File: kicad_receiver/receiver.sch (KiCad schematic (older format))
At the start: 59 parts, among them J1 Conn_01x05_Male, J2 Conn_01x01, J3 Conn_01x01, J4 Conn_01x01, J5 Conn_01x01, J6 Conn_01x01, J7 Conn_01x01, U1 LP2985-3.3, U10 L9110, U11 4N26, U12 4N26, U2 LP2985-3.3, U3 STM32F030F4Px, U4 NRF24L01_Breakout, U5 TP4056, U6 L9110, U7 MT3608, U8 4N26, U9 4N26

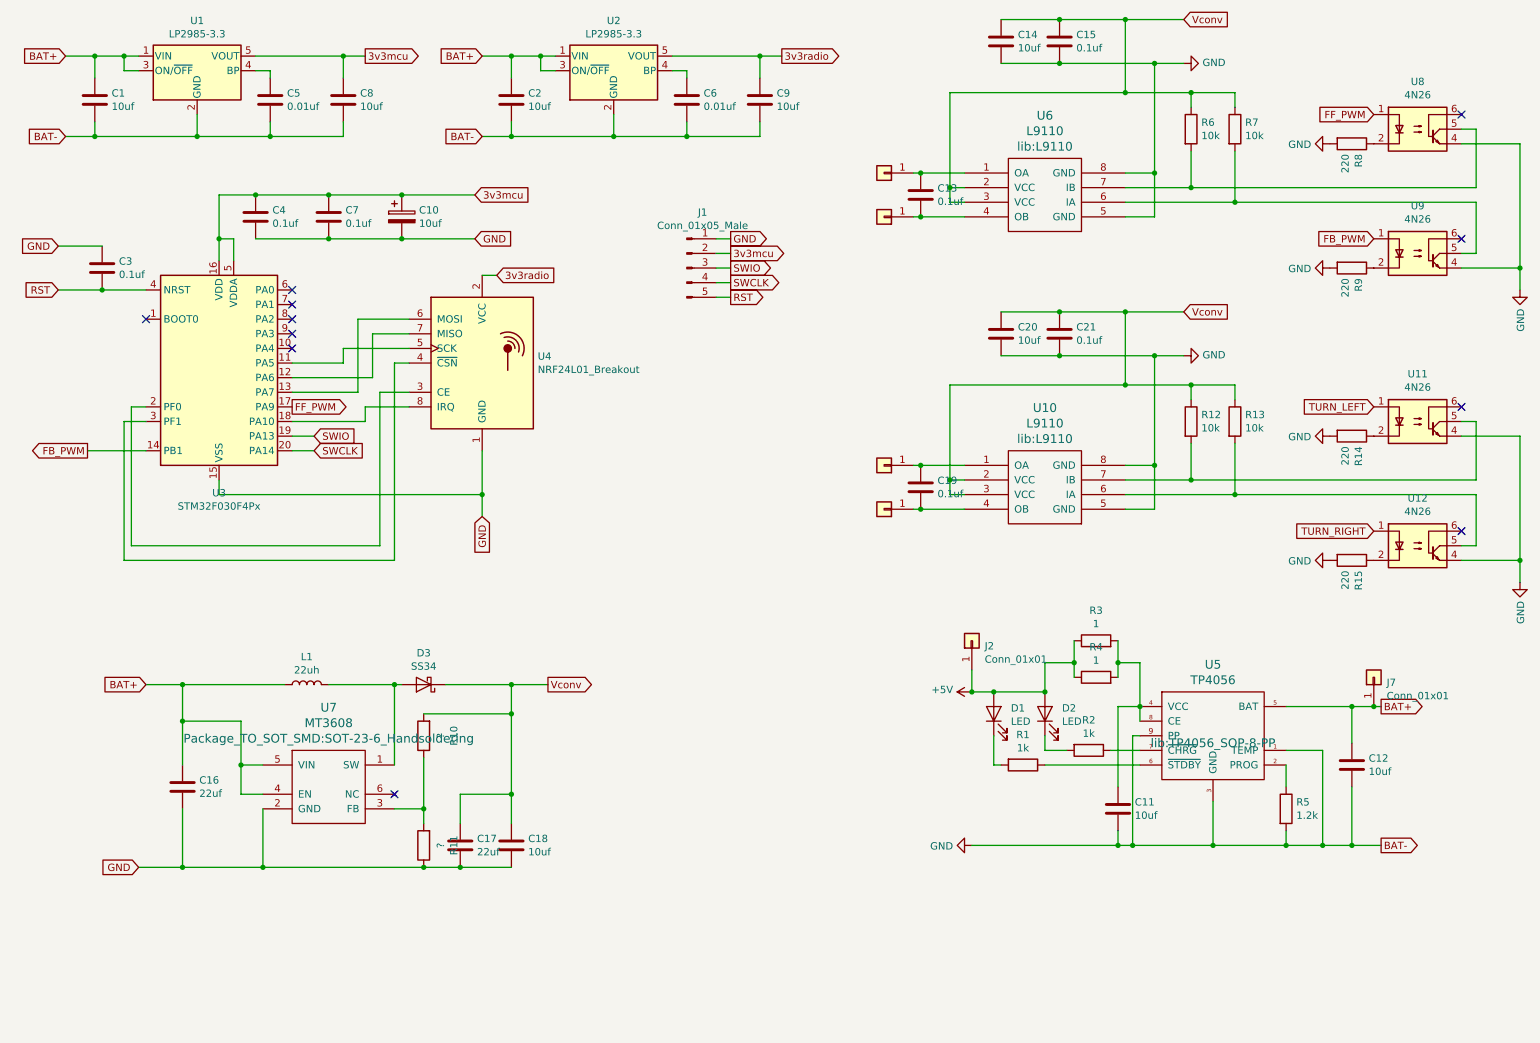
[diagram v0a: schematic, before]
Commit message: refactored
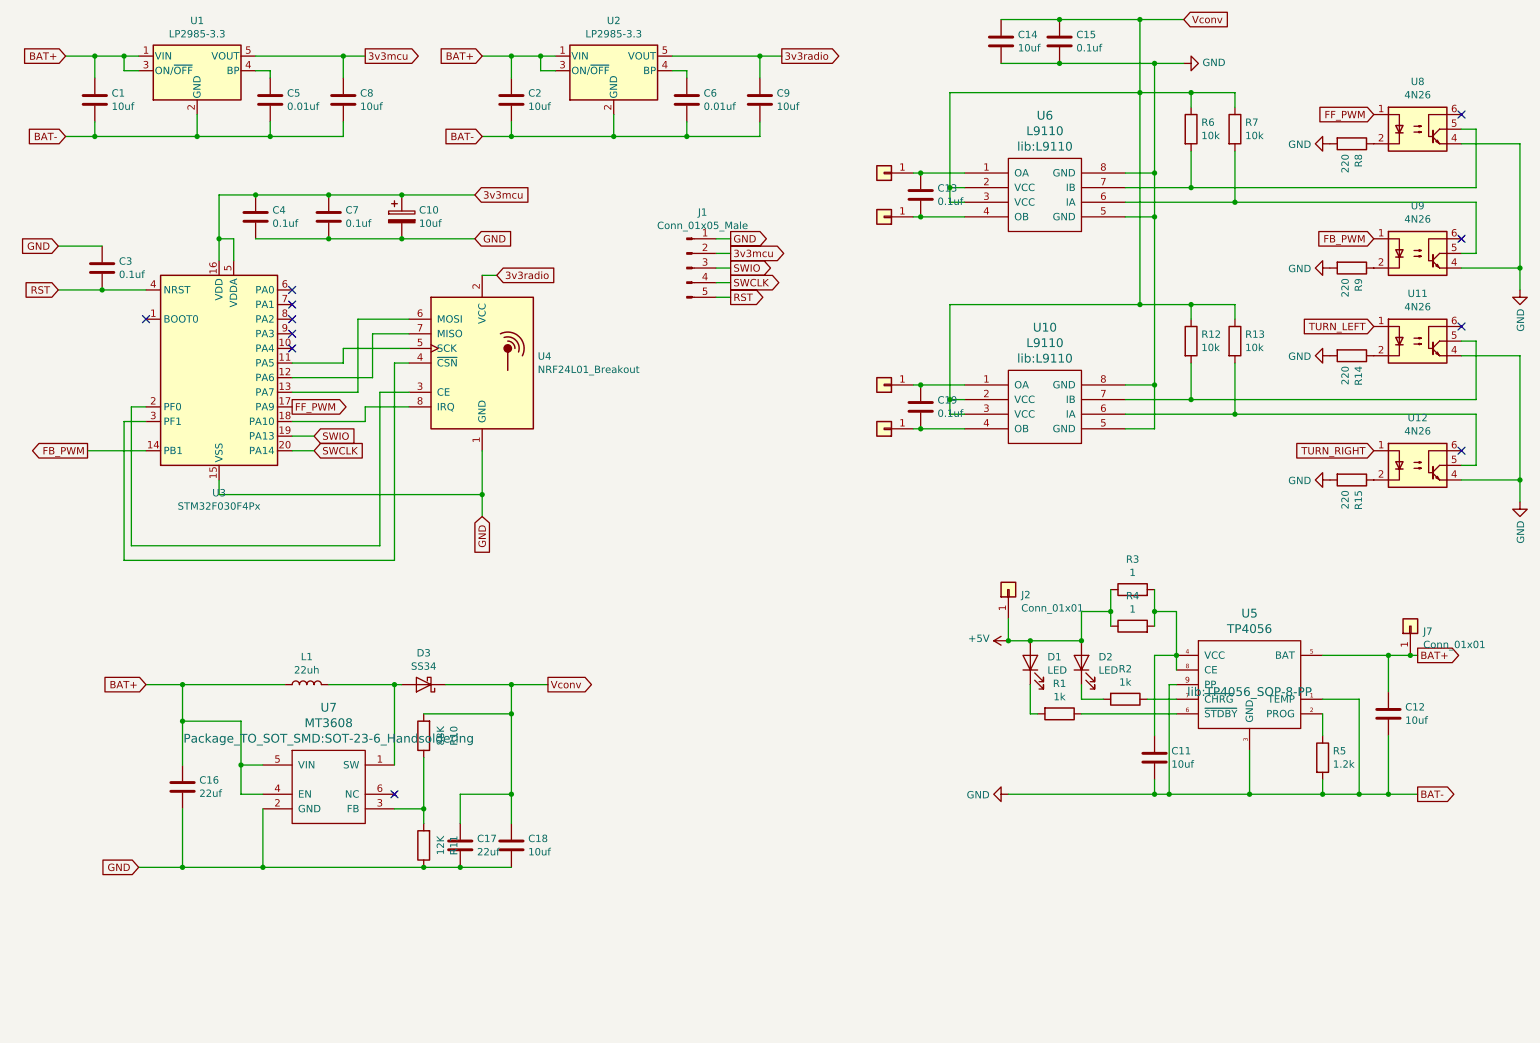
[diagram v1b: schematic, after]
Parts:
- removed C20: 10uf, Capacitor_SMD:C_0603_1608Metric_Pad1.05x0.95mm_HandSolder, symbol Device:C
- removed C21: 0.1uf, Capacitor_SMD:C_0603_1608Metric_Pad1.05x0.95mm_HandSolder, symbol Device:C
- R10: value ? -> 88K
- R11: value ? -> 12K
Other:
- moved on the sheet: C11, C12, C19, D1, D2, J2, J7, R1, R12, R13, R14, R15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

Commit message: place done
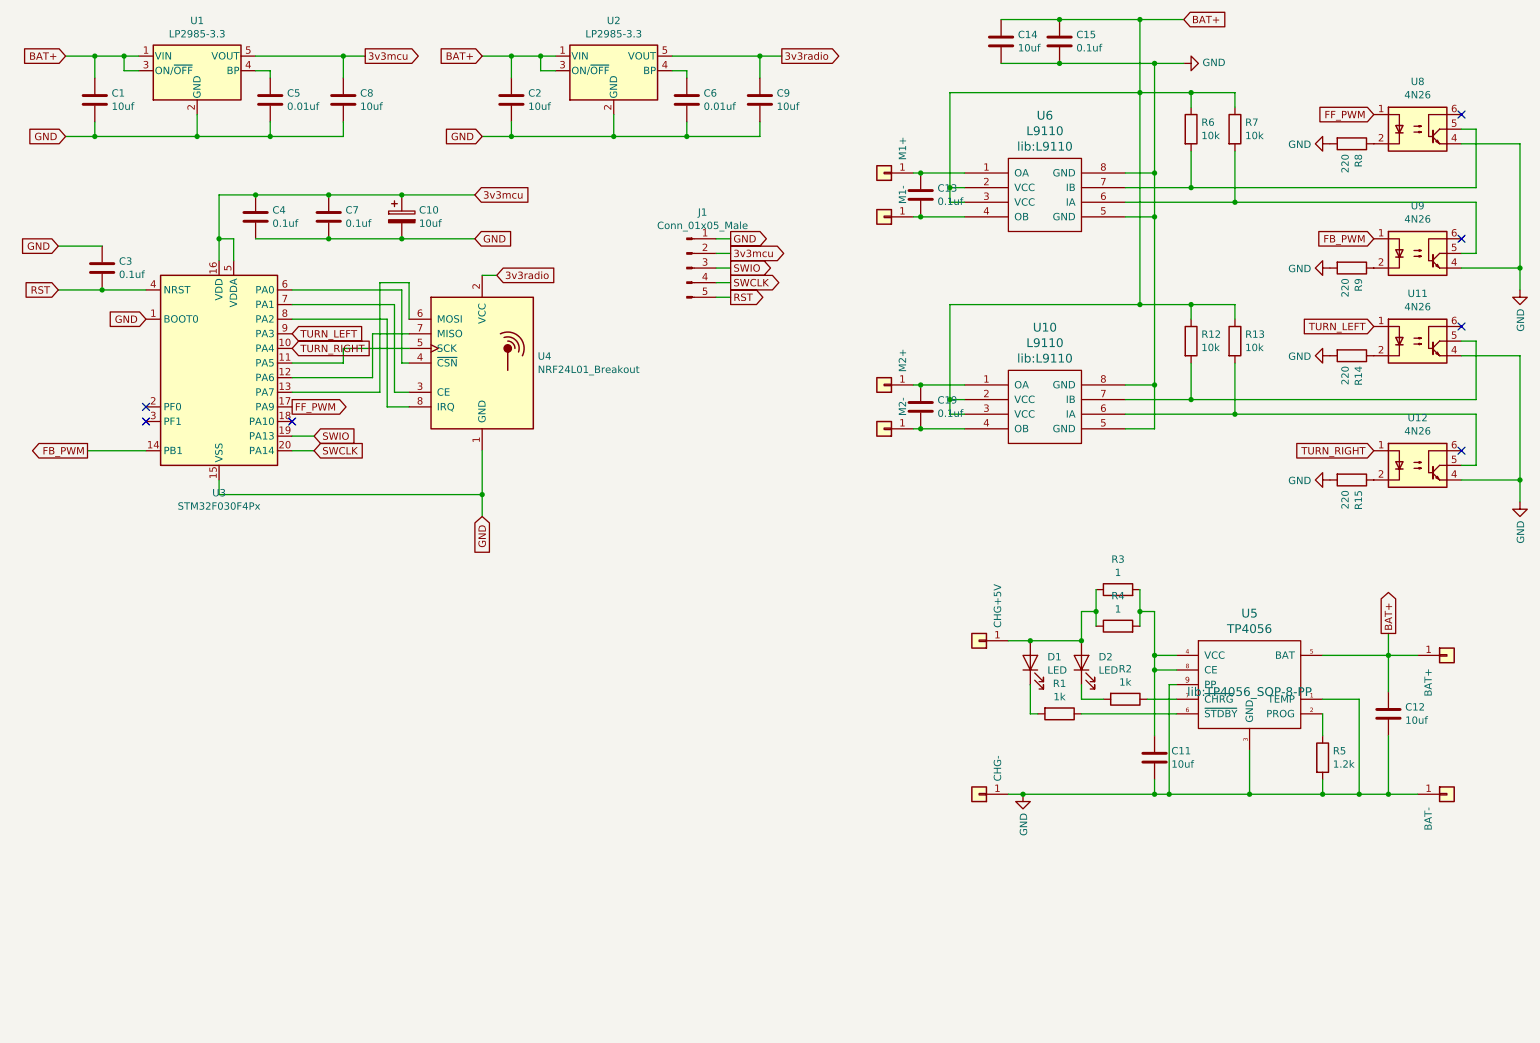
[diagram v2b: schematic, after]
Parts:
- removed C16, C17: 22uf, Capacitor_SMD:C_0805_2012Metric_Pad1.15x1.40mm_HandSolder, symbol Device:C
- removed C18: 10uf, Capacitor_SMD:C_0805_2012Metric_Pad1.15x1.40mm_HandSolder, symbol Device:C
- removed D3: SS34, Diode_SMD:D_2114_3652Metric, symbol Device:D_Schottky
- removed L1: 22uh, Inductor_SMD:L_10.4x10.4_H4.8, symbol Device:L
- removed R10: 88K, Resistor_SMD:R_0603_1608Metric_Pad1.05x0.95mm_HandSolder, symbol Device:R
- removed R11: 12K, Resistor_SMD:R_0603_1608Metric_Pad1.05x0.95mm_HandSolder, symbol Device:R
- removed U7: MT3608, Package_TO_SOT_SMD:SOT-23-6_Handsoldering, symbol mt3608:MT3608
- added J8: BAT+, TestPoint:TestPoint_Pad_4.0x4.0mm, symbol Connector_Generic:Conn_01x01
- added J9: BAT-, TestPoint:TestPoint_Pad_4.0x4.0mm, symbol Connector_Generic:Conn_01x01
- J2: value Conn_01x01 -> CHG+5V; footprint Connector_Wire:SolderWirePad_1x01_SMD_5x10mm -> TestPoint:TestPoint_Pad_4.0x4.0mm
- J3: value Conn_01x01 -> M1+; footprint Connector_Wire:SolderWirePad_1x01_SMD_5x10mm -> TestPoint:TestPoint_Pad_4.0x4.0mm
- J4: value Conn_01x01 -> M1-; footprint Connector_Wire:SolderWirePad_1x01_SMD_5x10mm -> TestPoint:TestPoint_Pad_4.0x4.0mm
- J5: value Conn_01x01 -> M2+; footprint Connector_Wire:SolderWirePad_1x01_SMD_5x10mm -> TestPoint:TestPoint_Pad_4.0x4.0mm
- J6: value Conn_01x01 -> M2-; footprint Connector_Wire:SolderWirePad_1x01_SMD_5x10mm -> TestPoint:TestPoint_Pad_4.0x4.0mm
- J7: value Conn_01x01 -> CHG-; footprint Connector_Wire:SolderWirePad_1x01_SMD_5x10mm -> TestPoint:TestPoint_Pad_4.0x4.0mm
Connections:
- net Vconv is gone; now on net BAT+: C14.1, C15.1, R12.1, R13.1, R6.1, R7.1, U10.2 (VCC), U10.3 (VCC), U6.2 (VCC), U6.3 (VCC)
- net BAT+: now also J8.1 (Pin_1); no longer J7.1 (Pin_1)
- net GND: now also J7.1 (Pin_1), U3.1 (BOOT0), J9.1 (Pin_1)
- net TURN_LEFT: now also U3.9 (PA3)
- net TURN_RIGHT: now also U3.10 (PA4)
- net at U4.3 (CE): now also U3.7 (PA1); no longer U3.2 (PF0)
- net at U4.4 (~CSN): now also U3.6 (PA0); no longer U3.3 (PF1)
- net at U4.8 (IRQ): now also U3.8 (PA2); no longer U3.18 (PA10)
- net +5V: no longer names the net of D1.2 (A), D2.2 (A), J2.1 (Pin_1), R3.1, R4.1
- no-connect marks 11 -> 7
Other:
- moved on the sheet: R3, R4

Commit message: fixed
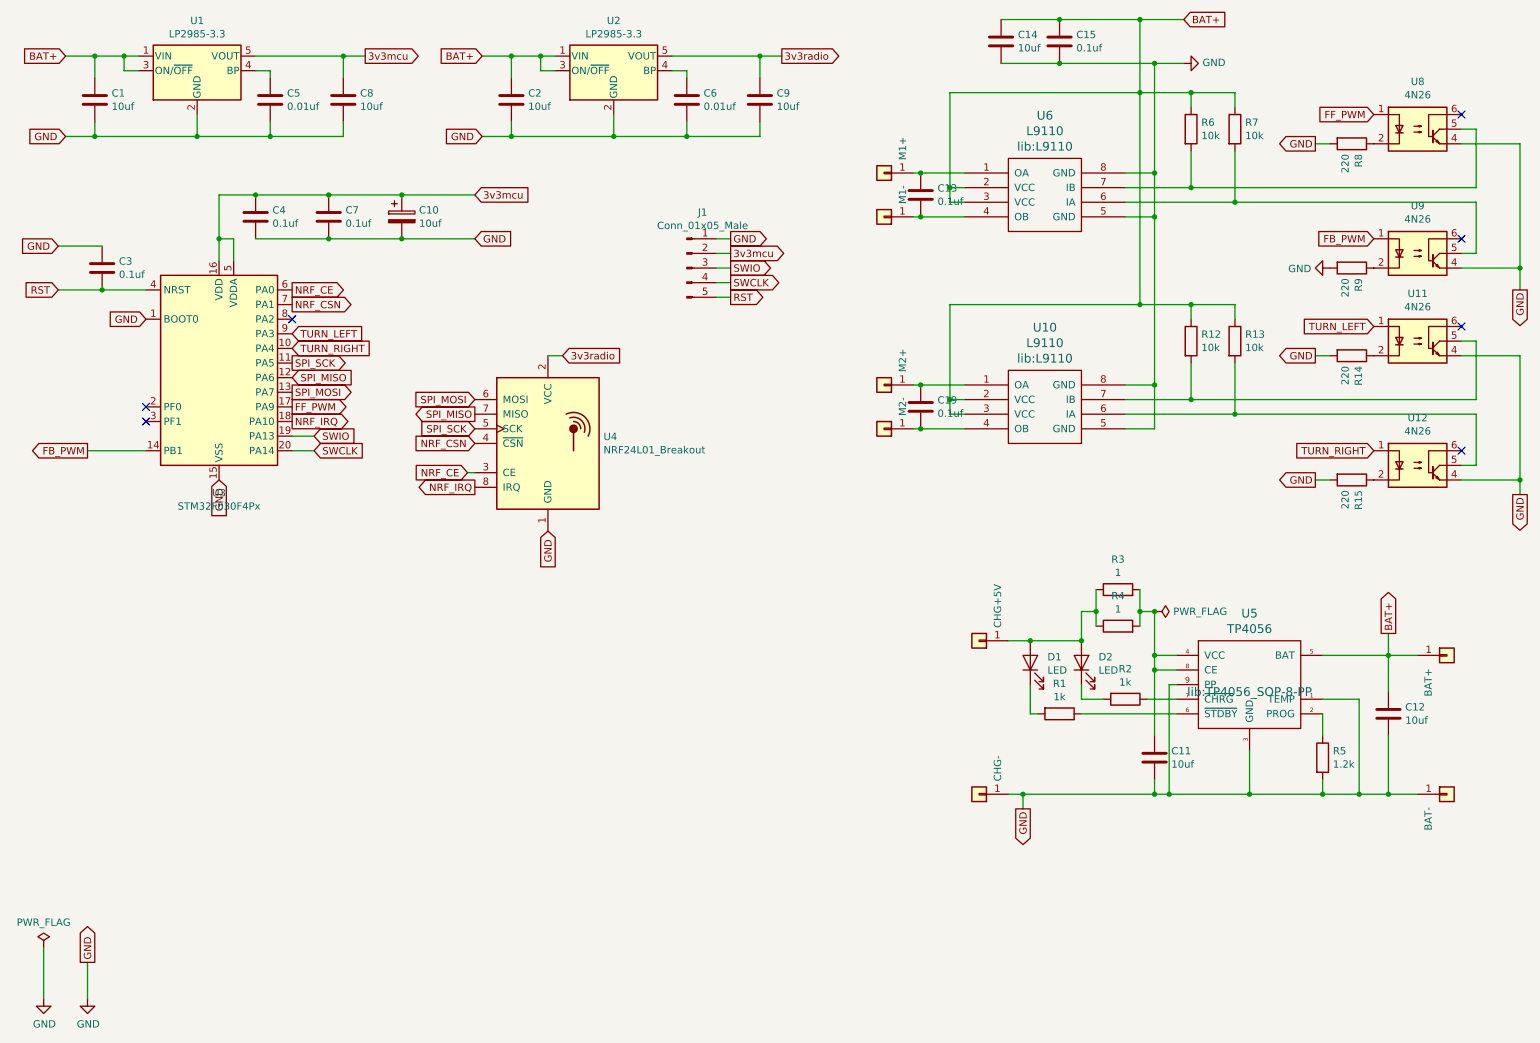
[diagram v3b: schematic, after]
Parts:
- C1, C11, C12, C13, C14, C15, C19, C2, C4, C5, C6, C7, C8, C9: footprint Capacitor_SMD:C_0603_1608Metric_Pad1.05x0.95mm_HandSolder -> Capacitor_SMD:C_0805_2012Metric_Pad1.15x1.40mm_HandSolder
- J2, J3, J4, J5, J6, J7, J8, J9: footprint TestPoint:TestPoint_Pad_4.0x4.0mm -> TestPoint:TestPoint_Pad_2.5x2.5mm
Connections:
- net NRF_CE: now reaches U4.3 (CE)
- net NRF_CE: now also U3.6 (PA0); no longer U3.7 (PA1)
- net NRF_CSN: now reaches U4.4 (~CSN)
- net NRF_CSN: now also U3.7 (PA1); no longer U3.6 (PA0)
- net SPI_SCK: now reaches U3.11 (PA5), U4.5 (SCK)
- net SPI_MOSI: now reaches U3.13 (PA7), U4.6 (MOSI)
- net SPI_MISO: now reaches U3.12 (PA6), U4.7 (MISO)
- net at U3.8 (PA2): no longer U4.8 (IRQ)
- net NRF_IRQ: now reaches U3.18 (PA10)
- net NRF_IRQ: now also U4.8 (IRQ)
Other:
- moved on the sheet: U4

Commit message: refactored
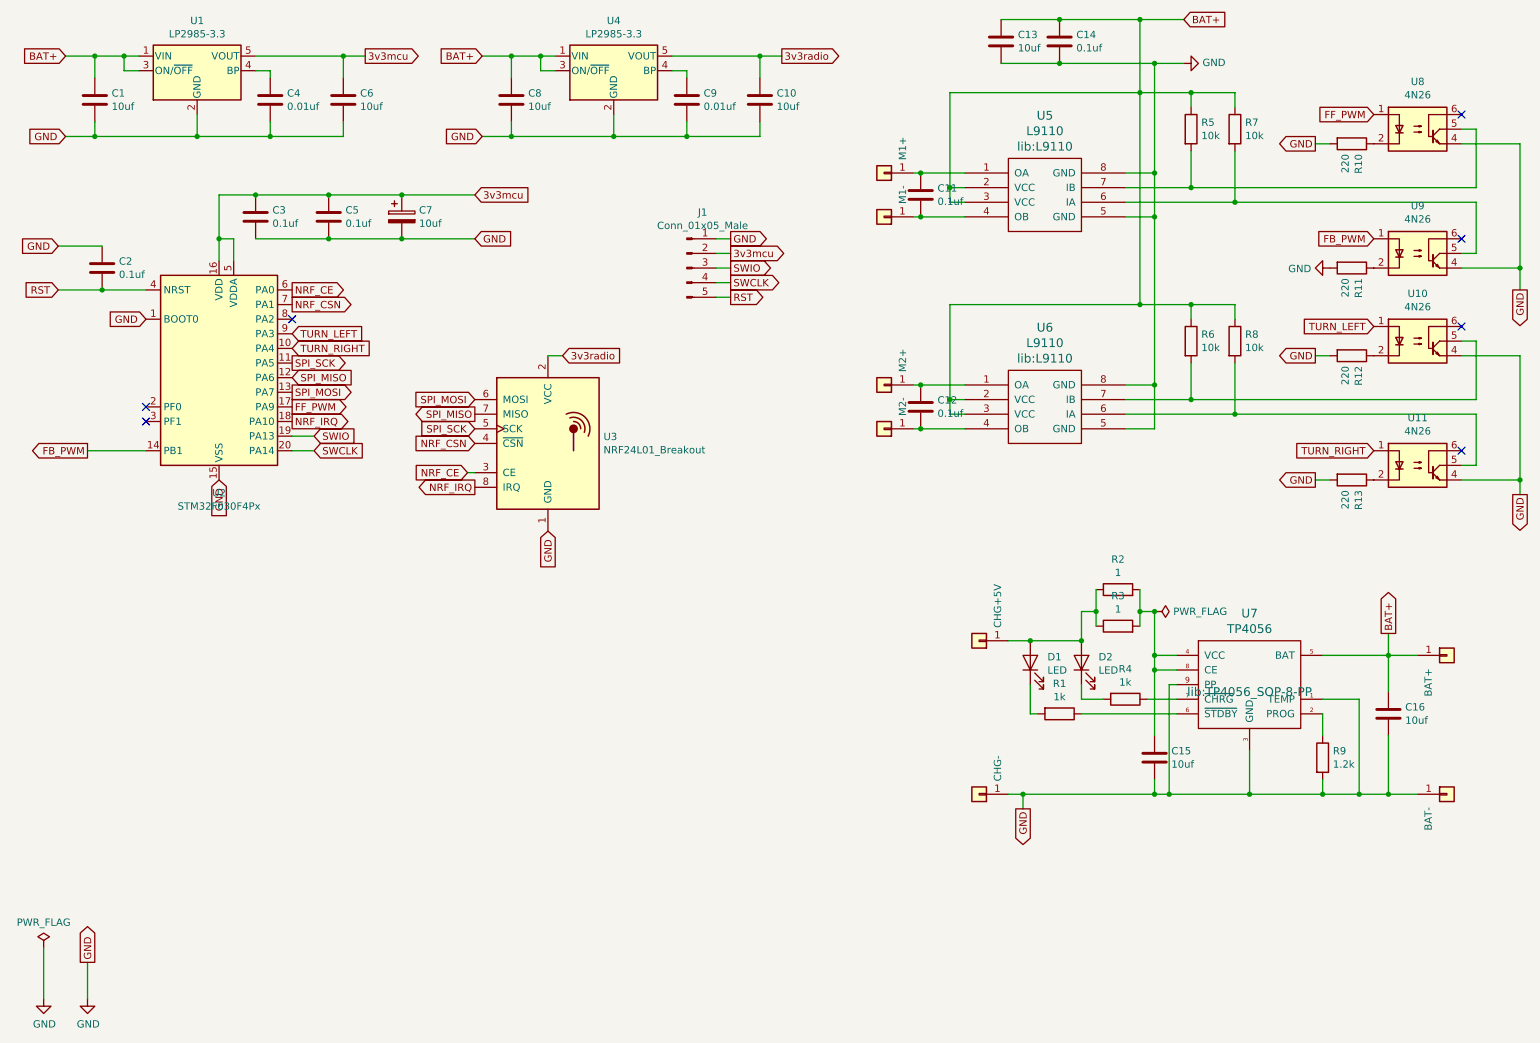
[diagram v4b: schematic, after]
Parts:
- renumbered C9 to C10, C13 to C11, C19 to C12, C14 to C13, C15 to C14, C11 to C15, C12 to C16, C3 to C2, C4 to C3, C5 to C4, C7 to C5, C8 to C6, C10 to C7, C2 to C8, C6 to C9, J3 to J2, J4 to J3, J5 to J4, J6 to J5, J2 to J6, R8 to R10, R9 to R11, R14 to R12, R15 to R13, R3 to R2, R4 to R3, R2 to R4, R6 to R5, R12 to R6, R13 to R8, R5 to R9, U11 to U10, U12 to U11, U3 to U2, U4 to U3, U2 to U4, U6 to U5, U10 to U6, U5 to U7
